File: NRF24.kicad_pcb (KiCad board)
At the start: 4 copper layers, 35.9 x 36.4 mm, 41 parts, among them J1 Conn_ARM_JTAG_SWD_10, J2 SMA, Q1 PMF170XP, Q2 PMF170XP, U1 Si7021-A20, U2 STM32L031G6Ux, U3 nRF24L01P, Y1 16MHz

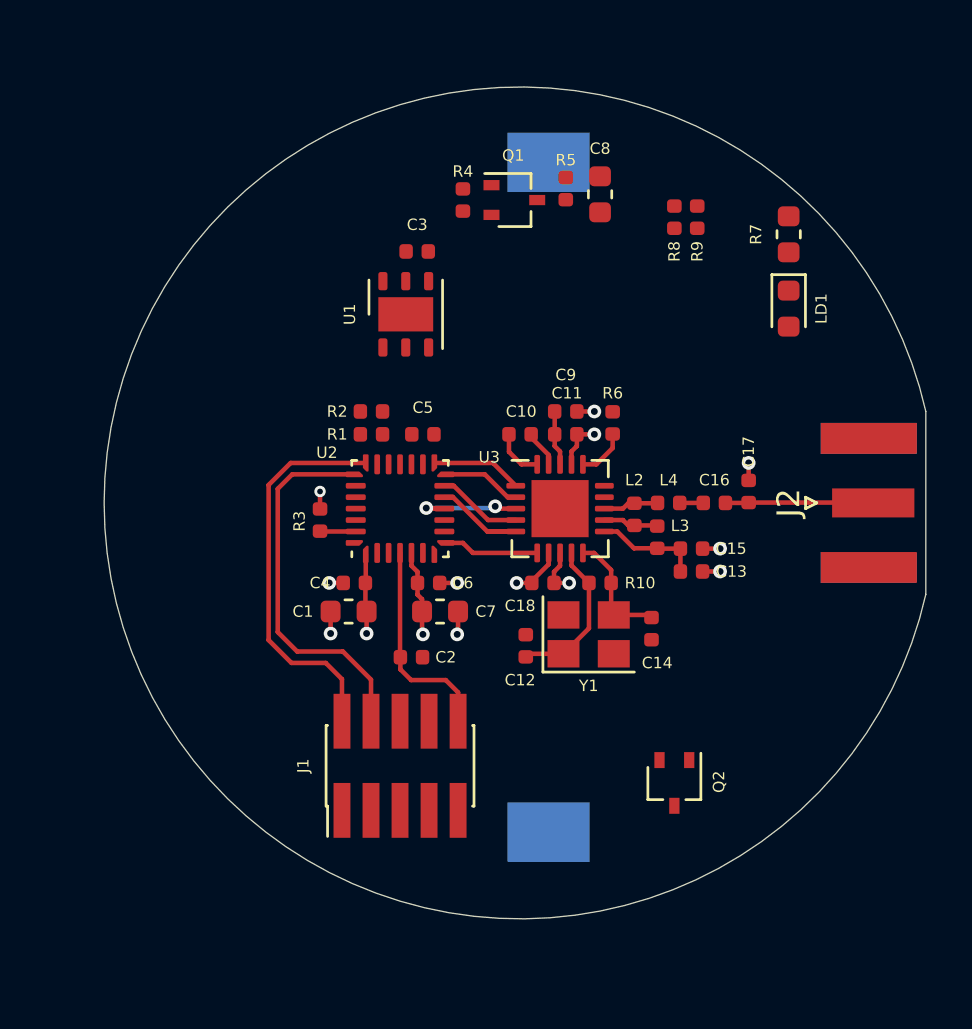
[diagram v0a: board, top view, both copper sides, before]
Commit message: Layout
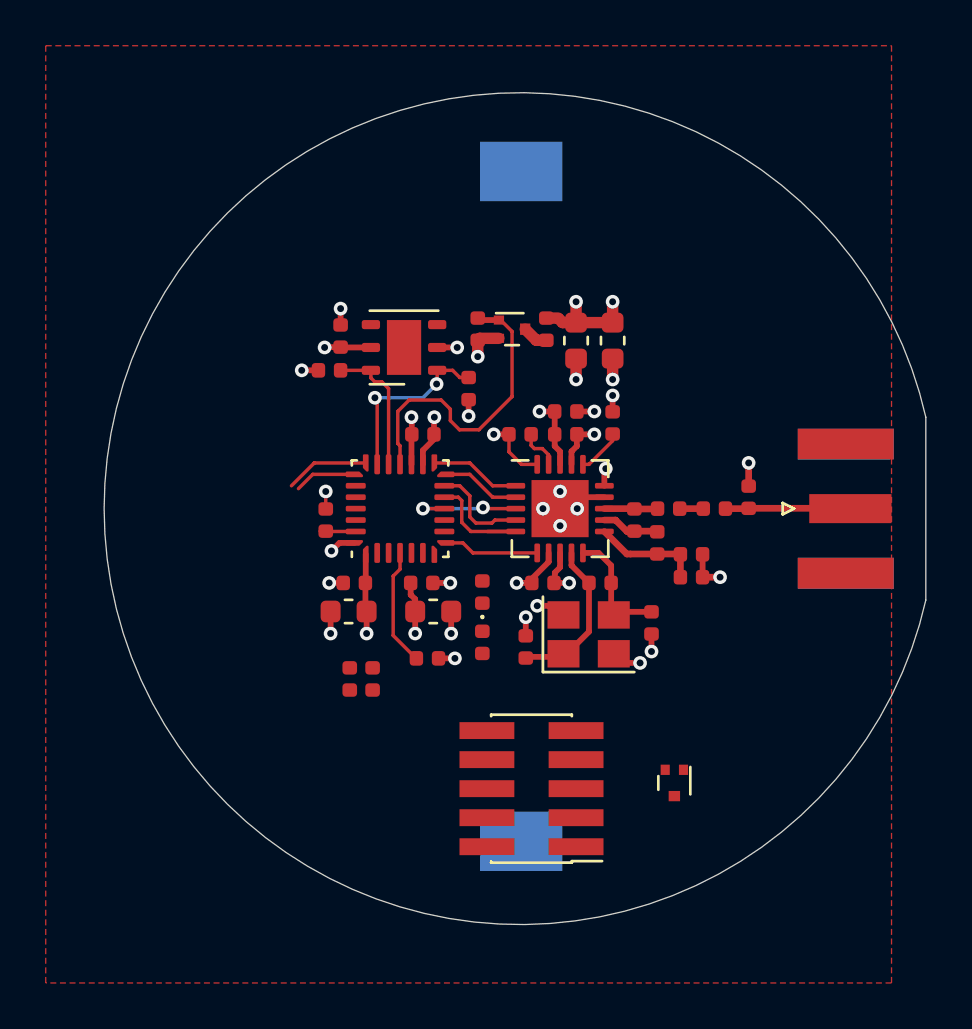
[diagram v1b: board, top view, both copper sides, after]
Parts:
- added C19: TBD, Capacitor_SMD:C_0603_1608Metric, F.Cu at (184.8, 79.9)
- LD1: value GREEN -> BLUE; footprint LED_SMD:LED_0603_1608Metric -> LED_SMD:LED_0402_1005Metric
- Q1, Q2: value PMF170XP -> NTK3139P; footprint Package_TO_SOT_SMD:SOT-323_SC-70 -> Package_TO_SOT_SMD:SOT-723
- R7: value 2k2 -> 10R; footprint Resistor_SMD:R_0603_1608Metric -> Resistor_SMD:R_0402_1005Metric
- moved R8 24.7 mm to (173.3, 94.7)
- moved R9 24.7 mm to (174.3, 94.7)
- moved R7 22.3 mm to (179.1, 93.1), turned to 270 degrees
- moved LD1 18.3 mm to (179.1, 90.9), turned to 90 degrees
- moved C8 6.49 mm to (183.2, 79.9)
- moved R5 6.21 mm to (181.9, 79.4)
- moved J1 5.84 mm to (181.2, 99.5), turned to 180 degrees
- moved R4 5.69 mm to (178.9, 79.4)
- moved Q1 5.65 mm to (180.4, 79.4)
- moved C3 4.99 mm to (172.9, 79.7), turned to 90 degrees
- moved R2 4.37 mm to (178.5, 82.0), turned to 90 degrees
- moved R1 3.35 mm to (172.4, 81.2)
- moved U1 1.45 mm to (175.7, 80.2), turned to 180 degrees
- moved BT1 1.26 mm to (180.8, 87.2)
- moved J2 1.03 mm to (195.0, 87.2)
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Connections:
- U3 pad 21: (no net) -> GND
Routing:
- net GND: track 13.7 -> 29.3 mm, vias 11 -> 27
- net /SWCLK: track 16.6 -> 2.71 mm
- net /NRF_PWR: track 0.00 -> 13.6 mm
- net /SWDIO: track 17.2 -> 3.66 mm
- net /I2C_SDA: track 0.00 -> 8.02 mm, vias 0 -> 2
- net VCC: track 7.32 -> 14.4 mm, vias 2 -> 7
- net +VSW: track 4.69 -> 10.9 mm, vias 1 -> 5
- net /I2C_SCL: track 0.00 -> 5.94 mm
- net /NRST: track 9.30 -> 5.17 mm
- net Net-(Q1-Pad3): track 0.00 -> 1.13 mm
- net Net-(C16-Pad1): track 6.48 -> 5.50 mm
- net /SPI_MOSI: track 3.75 -> 4.40 mm
- net /SPI_MISO: track 4.99 -> 5.54 mm
- added copper zone on F.Cu, net GND
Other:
- net class Default: clearance 0.15 -> 0.2; trace_width 0.15 -> 0.1524; via_dia 0.8 -> 0.6; via_drill 0.4 -> 0.3
- rule trace_clearance: 0.15 -> 0.2
- rule trace_min: 0.1 -> 0.152

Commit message: Layout
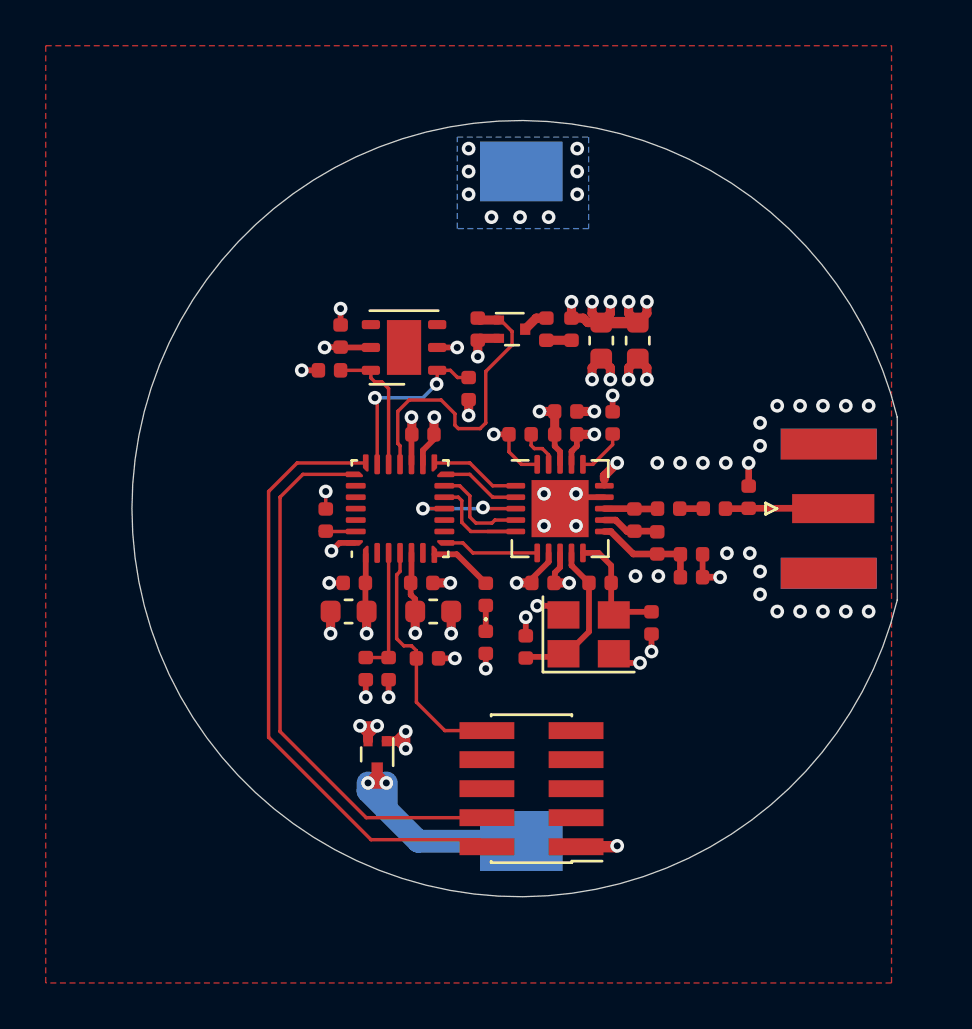
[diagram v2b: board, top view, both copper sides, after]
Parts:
- added BT1: CR2032, Battery:BatteryHolder_Keystone_1060_1x2032, B.Cu at (180.8, 87.2)
- added FB1: 100 @ 100MHz, Inductor_SMD:L_0402_1005Metric, F.Cu at (181.9, 79.4)
- moved Q2 13.1 mm to (174.5, 98.0)
- moved C8 1.10 mm to (184.3, 79.9)
- moved C19 1.10 mm to (185.9, 79.9)
- moved R5 1.10 mm to (183.0, 79.4)
- moved R8 0.83 mm to (174.0, 94.2)
- moved R9 0.83 mm to (175.0, 94.2)
- moved J2 0.75 mm to (194.2, 87.2)
- moved LD1 0.18 mm to (179.2, 91.0)
- moved R7 0.15 mm to (179.2, 93.1)
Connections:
- Q1 pad 3: Net-(Q1-Pad3) -> Net-(FB1-Pad2)
- R5 pad 2: Net-(Q1-Pad3) -> Net-(FB1-Pad1)
- U2 pad 3: Net-(U2-Pad3) -> /BAT_LEVEL
- U2 pad 6: /LED_STATUS -> Net-(U2-Pad6)
- U2 pad 7: /BAT_LEVEL -> /LED_STATUS
- U3 pad 21: GND -> (no net)
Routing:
- net /SWDIO: track 3.66 -> 27.1 mm
- net /SWCLK: track 2.71 -> 24.5 mm
- net Net-(BT1-Pad1): track 0.00 -> 11.3 mm, vias 0 -> 2
- net GND: track 29.3 -> 36.0 mm, vias 27 -> 64
- net VCC: track 14.4 -> 20.7 mm, vias 7 -> 11
- net /NRST: track 5.17 -> 10.7 mm
- net /BAT_LEVEL: track 0.00 -> 5.33 mm
- net +VSW: track 10.9 -> 14.6 mm, vias 5 -> 8
- net /LED_STATUS: track 0.00 -> 2.78 mm
- net Net-(LD1-Pad1): track 0.00 -> 1.13 mm
- net Net-(Q1-Pad3): track 1.13 -> 0.00 mm
- net Net-(FB1-Pad2): track 0.00 -> 1.13 mm
- net Net-(FB1-Pad1): track 0.00 -> 1.10 mm
- added copper zone on B.Cu, net GND
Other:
- board size 35.9 x 36.4 mm -> 33.5 x 34 mm
